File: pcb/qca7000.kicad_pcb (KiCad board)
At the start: 4 copper layers, 41.6 x 28.2 mm, 111 parts, among them J1 Conn_01x20, J2 JTAG, J3 FLASH, U1 25Q16, Y1 25MHz

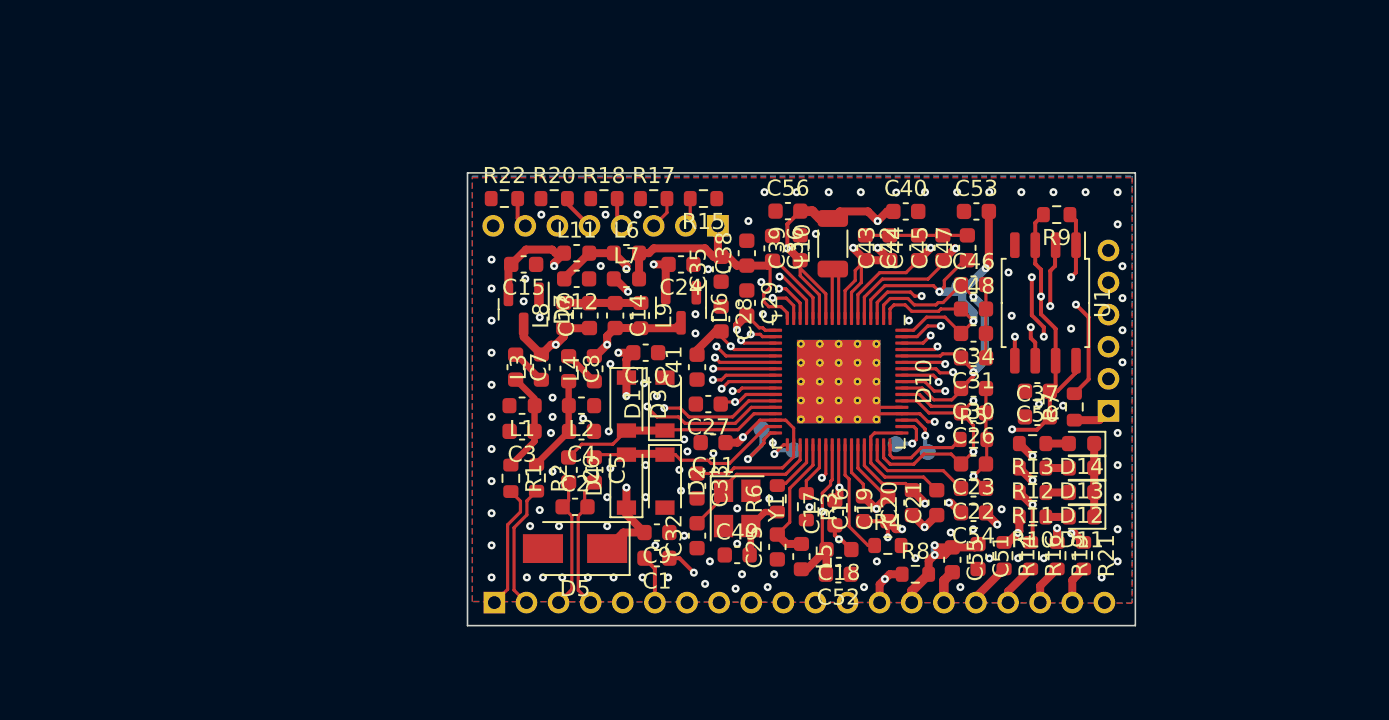
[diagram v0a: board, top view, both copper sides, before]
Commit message: schematic improvements and board draft
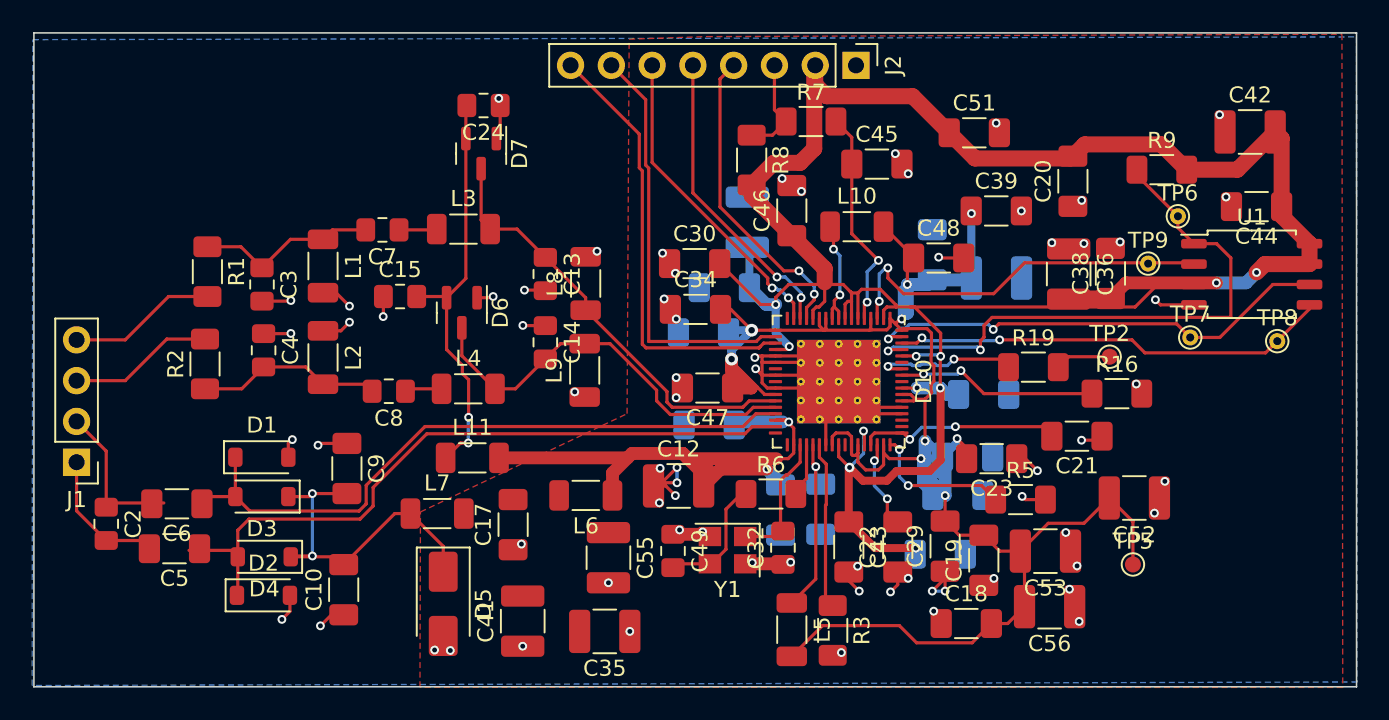
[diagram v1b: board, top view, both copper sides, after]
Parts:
- removed C1: 100nF, Capacitor_SMD:C_0603_1608Metric
- removed D11, D12, D13, D14: 19-217/GHC-YR1S2/3T, LED_SMD:LED_0603_1608Metric
- removed J3: FLASH, Connector_PinSocket_2.00mm:PinSocket_1x06_P2.00mm_Vertical
- removed R10, R11, R12, R13, R14, R18, R21: 3.3K, Resistor_SMD:R_0603_1608Metric
- removed R15, R17, R20, R22, R4: 10k, Resistor_SMD:R_0603_1608Metric
- removed TP1, TP3, TP4: TestPoint, TestPoint:TestPoint_Pad_D1.0mm
- added TP6: FL_CS, TestPoint:TestPoint_THTPad_D1.0mm_Drill0.5mm, F.Cu at (156.8, 51.5)
- added TP7: FL_CLK, TestPoint:TestPoint_THTPad_D1.0mm_Drill0.5mm, F.Cu at (157.5, 59.0)
- added TP8: FL_MOSI, TestPoint:TestPoint_THTPad_D1.0mm_Drill0.5mm, F.Cu at (162.9, 59.3)
- added TP9: FL_MISO, TestPoint:TestPoint_THTPad_D1.0mm_Drill0.5mm, F.Cu at (154.9, 54.5)
- C10, C17, C18, C19, C20, C21, C22, C23, C29, C30, C34, C38, C39, C43, C44, C45, C46, C47, C48, C5, C51, C6, C9: footprint Capacitor_SMD:C_0603_1608Metric -> Capacitor_SMD:C_1206_3216Metric_Pad1.33x1.80mm_HandSolder
- C11, C16, C25, C26, C27, C28, C31, C33, C40, C50: footprint Capacitor_SMD:C_0603_1608Metric -> Capacitor_SMD:C_1206_3216Metric_Pad1.33x1.80mm_HandSolder; moved to B.Cu
- C12, C35, C36, C41, C42, C52, C53, C55, C56: value 10uF 25V -> 10uF 10V; footprint Capacitor_SMD:C_0603_1608Metric -> Capacitor_SMD:C_1210_3225Metric_Pad1.33x2.70mm_HandSolder
- C13, C14, C15, C2, C24, C3, C32, C4, C49, C7, C8: footprint Capacitor_SMD:C_0603_1608Metric -> Capacitor_SMD:C_0805_2012Metric_Pad1.18x1.45mm_HandSolder
- C37, C54: value 10uF 25V -> 10uF 10V; footprint Capacitor_SMD:C_0603_1608Metric -> Capacitor_SMD:C_1210_3225Metric_Pad1.33x2.70mm_HandSolder; moved to B.Cu
- J1: value Conn_01x20 -> Conn_01x04_Pin; footprint Connector_PinSocket_2.00mm:PinSocket_1x20_P2.00mm_Vertical -> Connector_PinHeader_2.54mm:PinHeader_1x04_P2.54mm_Vertical; moved to F.Cu
- J2: value JTAG -> Conn_01x08_Pin; footprint Connector_PinHeader_2.00mm:PinHeader_1x08_P2.00mm_Vertical -> Connector_PinHeader_2.54mm:PinHeader_1x08_P2.54mm_Vertical; moved to F.Cu
- L1, L11, L2, L3, L4, L5, L6, L7, L8, L9: footprint Inductor_SMD:L_0603_1608Metric -> Inductor_SMD:L_1206_3216Metric_Pad1.22x1.90mm_HandSolder
- L10: footprint Inductor_SMD:L_1206_3216Metric -> Inductor_SMD:L_1206_3216Metric_Pad1.22x1.90mm_HandSolder
- R1, R16, R19, R2, R6, R7, R8, R9: footprint Resistor_SMD:R_0603_1608Metric -> Resistor_SMD:R_1206_3216Metric_Pad1.30x1.75mm_HandSolder
- R3, R5: value R_Small -> 2.5k; footprint Resistor_SMD:R_0603_1608Metric -> Resistor_SMD:R_1206_3216Metric_Pad1.30x1.75mm_HandSolder
- TP2: value TestPoint -> GPIO_2R; moved to F.Cu
- TP5: value TestPoint -> 1V2; moved to F.Cu
- moved C56 29.5 mm to (148.8, 75.8), turned to 180 degrees
- moved C2 29.2 mm to (90.0, 70.7), turned to -90 degrees
- moved R8 27.7 mm to (130.2, 48.0), turned to -90 degrees
- moved J1 27.5 mm to (88.2, 66.8), turned to 180 degrees
- moved C5 26.6 mm to (94.2, 72.2), turned to 180 degrees
- moved C51 26.4 mm to (144.1, 46.3), turned to 0 degrees
- moved D2 26.0 mm to (99.8, 75.1), turned to 0 degrees
- moved D1 25.3 mm to (99.7, 66.5), turned to 0 degrees
- moved C42 25.0 mm to (161.2, 46.2), turned to 0 degrees
- moved C6 24.5 mm to (94.4, 69.4), turned to 180 degrees
- moved R7 24.2 mm to (133.9, 45.6), turned to 0 degrees
- moved C10 23.9 mm to (104.8, 74.8), turned to 90 degrees
- moved C35 23.7 mm to (121.0, 77.4), turned to 180 degrees
- moved D3 23.4 mm to (99.7, 69.0), turned to 180 degrees
- moved D4 23.0 mm to (99.8, 72.7), turned to 180 degrees
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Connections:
- C13 pad 2: Net-(C13-Pad2) -> GND
- C14 pad 1: Net-(C13-Pad2) -> GND
- D10 pad 14: SERIAL_IO_4 -> SERIAL_IO_4_MOSI
- D10 pad 15: SERIAL_IO_3 -> SERIAL_IO_3_MISO
- D10 pad 16: SERIAL_IO_2 -> SERIAL_IO_2_CS
- D10 pad 19: SERIAL_IO_1 -> SERIAL_IO_1_CLK
- D10 pad 20: SERIAL_IO_0 -> SERIAL_IO_0_INT
- D10 pad 22: TDI -> GND
- D10 pad 23: TCK -> GND
- D10 pad 24: TDO -> unconnected-(D10-TDO-Pad24)
- D10 pad 25: TMS -> GND
- D10 pad 26: RTCK -> unconnected-(D10-RTCK-Pad26)
- D10 pad 27: TRST_L -> GND
- D10 pad 34: Net-(D10-Pad34) -> unconnected-(D10-ATB_N-Pad34)
- D10 pad 35: Net-(D10-Pad35) -> unconnected-(D10-ATB_P-Pad35)
- D10 pad 41: ZC -> GND
- D10 pad 44: Net-(D10-Pad44) -> unconnected-(D10-PLL_BYPASS-Pad44)
- D10 pad 53: Net-(D10-Pad53) -> unconnected-(D10-RSVD06-Pad53)
- D10 pad 54: Net-(D10-Pad54) -> unconnected-(D10-RSVD07-Pad54)
- D10 pad 60: GPIO_0 -> unconnected-(D10-GPIO_0-Pad60)
- D10 pad 63: GPIO_3 -> unconnected-(D10-GPIO_3-Pad63)
- J1 pad 1: RX_N -> TX_P
- J1 pad 2: RX_P -> TX_N
- J1 pad 3: TX_N -> RX_P
- J1 pad 4: TX_P -> RX_N
- J2 pad 1: +3V3_D -> GND
- J2 pad 2: TDI -> +3V3_D
- J2 pad 3: TCK -> RESET#
- J2 pad 4: TDO -> SERIAL_IO_4_MOSI
- J2 pad 5: TMS -> SERIAL_IO_3_MISO
- J2 pad 6: RTCK -> SERIAL_IO_2_CS
- J2 pad 7: TRST_L -> SERIAL_IO_1_CLK
- J2 pad 8: GND -> SERIAL_IO_0_INT
- L8 pad 2: Net-(C13-Pad2) -> GND
- L9 pad 1: Net-(C13-Pad2) -> GND
- R16 pad 2: Net-(J1-Pad17) -> GND
- R19 pad 2: Net-(J1-Pad18) -> Net-(R19-Pad2)
- TP2 pad 1: Net-(D10-Pad34) -> Net-(R19-Pad2)
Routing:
- net GND: track 45.2 -> 87.5 mm, vias 115 -> 71
- net +1V2_C: track 171.2 -> 134.4 mm, vias 12 -> 9
- net TXOUT_P: track 12.6 -> 44.1 mm
- net TXOUT_N: track 13.9 -> 42.6 mm
- net SERIAL_IO_0_INT: track 0.00 -> 27.8 mm
- net SERIAL_IO_4: track 26.3 -> 0.00 mm, vias 1 -> 0
- net SERIAL_IO_1_CLK: track 0.00 -> 26.2 mm
- net TRST_L: track 24.9 -> 0.00 mm, vias 1 -> 0
- net SERIAL_IO_3: track 23.1 -> 0.00 mm, vias 1 -> 0
- net RESET#: track 28.2 -> 6.30 mm, vias 1 -> 0
- net SERIAL_IO_2: track 21.6 -> 0.00 mm, vias 1 -> 0
- net GPIO_3: track 21.0 -> 0.00 mm, vias 3 -> 0
- net TMS: track 21.0 -> 0.00 mm, vias 1 -> 0
- net RTCK: track 20.5 -> 0.00 mm, vias 1 -> 0
- net +3V3_A: track 32.5 -> 52.7 mm
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- added copper zone on F.Cu, net +3V3_D
- removed copper zone on F.Cu, net GND
- removed copper zone on In1.Cu, net GND
- removed copper zone on In2.Cu, net GND
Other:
- board size 41.6 x 28.2 mm -> 82.4 x 40.7 mm

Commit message: board: more width for supply, fill, shrink
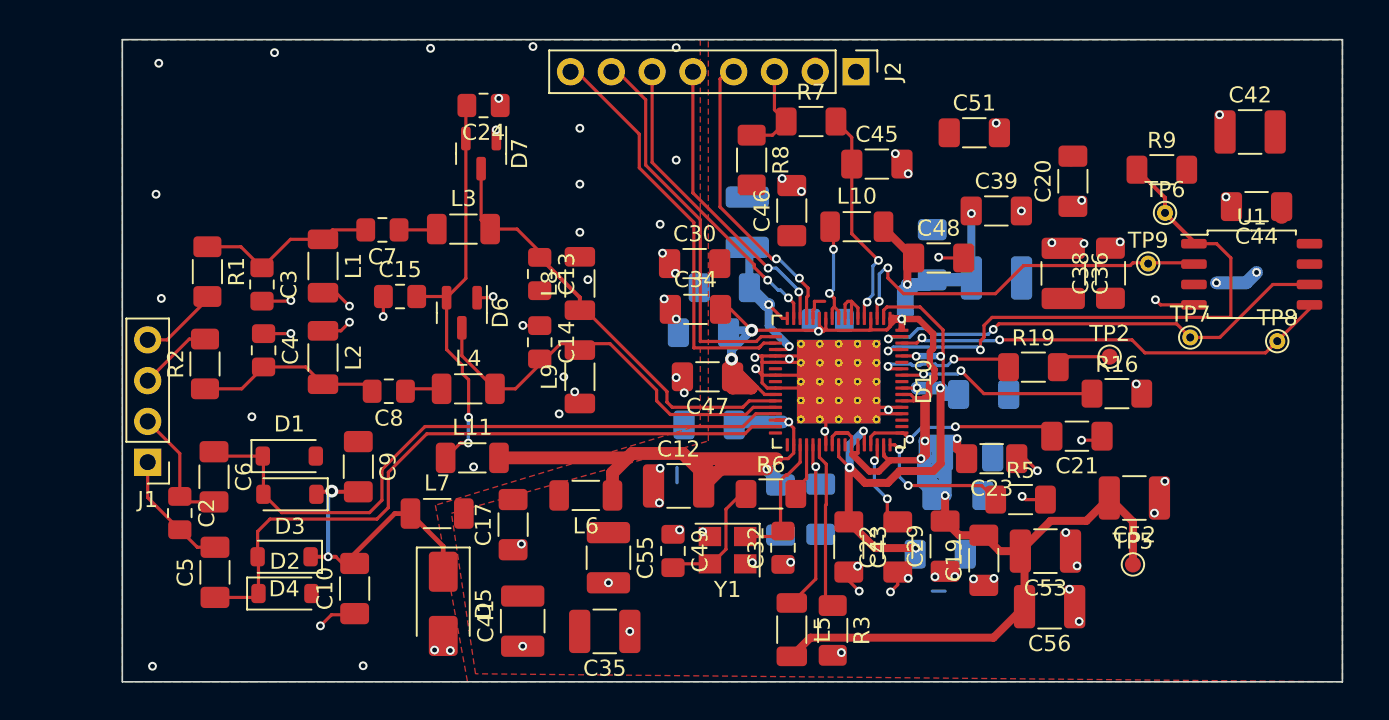
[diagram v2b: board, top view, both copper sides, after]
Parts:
- C18: footprint Capacitor_SMD:C_1206_3216Metric_Pad1.33x1.80mm_HandSolder -> Capacitor_SMD:C_0805_2012Metric_Pad1.18x1.45mm_HandSolder; moved to B.Cu
- moved C18 20.8 mm to (134.9, 58.0), turned to 180 degrees
- moved C2 4.63 mm to (94.6, 70.0)
- moved J1 4.43 mm to (92.6, 66.8)
- moved C5 2.92 mm to (96.8, 73.7), turned to 90 degrees
- moved C6 2.86 mm to (96.7, 67.7), turned to -90 degrees
- moved D3 1.75 mm to (101.4, 68.8)
- moved D1 1.71 mm to (101.4, 66.4)
- moved D2 1.34 mm to (101.1, 75.0)
- moved D4 1.24 mm to (101.1, 72.7)
- moved TP6 0.83 mm to (155.9, 51.3)
- moved C9 0.72 mm to (105.7, 67.1)
- moved C47 0.70 mm to (127.5, 61.5)
- moved C10 0.68 mm to (105.5, 74.7)
- moved L9 0.50 mm to (119.5, 61.5)
- moved J2 0.40 mm to (136.7, 42.5)
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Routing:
- net +3V3_D: track 170.7 -> 58.5 mm
- net GND: track 87.5 -> 64.0 mm, vias 71 -> 86
- net +1V2_C: track 134.4 -> 143.7 mm, vias 9 -> 10
- net RX_P: track 9.07 -> 4.64 mm
- net RX_N: track 9.27 -> 4.95 mm
- net Net-(D3-K): track 22.4 -> 19.1 mm
- net TX_N: track 9.80 -> 7.77 mm
- net SERIAL_IO_1_CLK: track 26.2 -> 24.3 mm
- net SERIAL_IO_0_INT: track 27.8 -> 26.1 mm
- net TX_P: track 9.27 -> 7.68 mm
- net TXOUT_P: track 44.1 -> 43.0 mm
- net TXOUT_N: track 42.6 -> 41.6 mm
- net SERIAL_IO_4_MOSI: track 19.3 -> 18.7 mm
- added copper zone on F.Cu, net GND
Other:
- board size 82.4 x 40.7 mm -> 76 x 40 mm
